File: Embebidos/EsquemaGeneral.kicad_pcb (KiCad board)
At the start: 2 copper layers, 100 x 99.9 mm, 79 parts, among them IC1 ESP32-WROVER-B__8MB_, J1 USB_A, J2 Conn_01x02, J3 RJ45, J4 RJ45, J5 Conn_02x06_Counter_Clockwise, J6 Conn_01x08, J7 Conn_01x04, Q1 BC847, Q2 BC847, Q3 BSS138, Q4 DMP3056LSDQ-13, Q5 BSS138, Q6 DMP3056LSDQ-13, SW1 SW_Reset, SW2 SW_Boot, U2 LM358, U3 SPX3819M5-L-3-3, U4 MIC29302WU, U5 MIC5219-3.3YM5

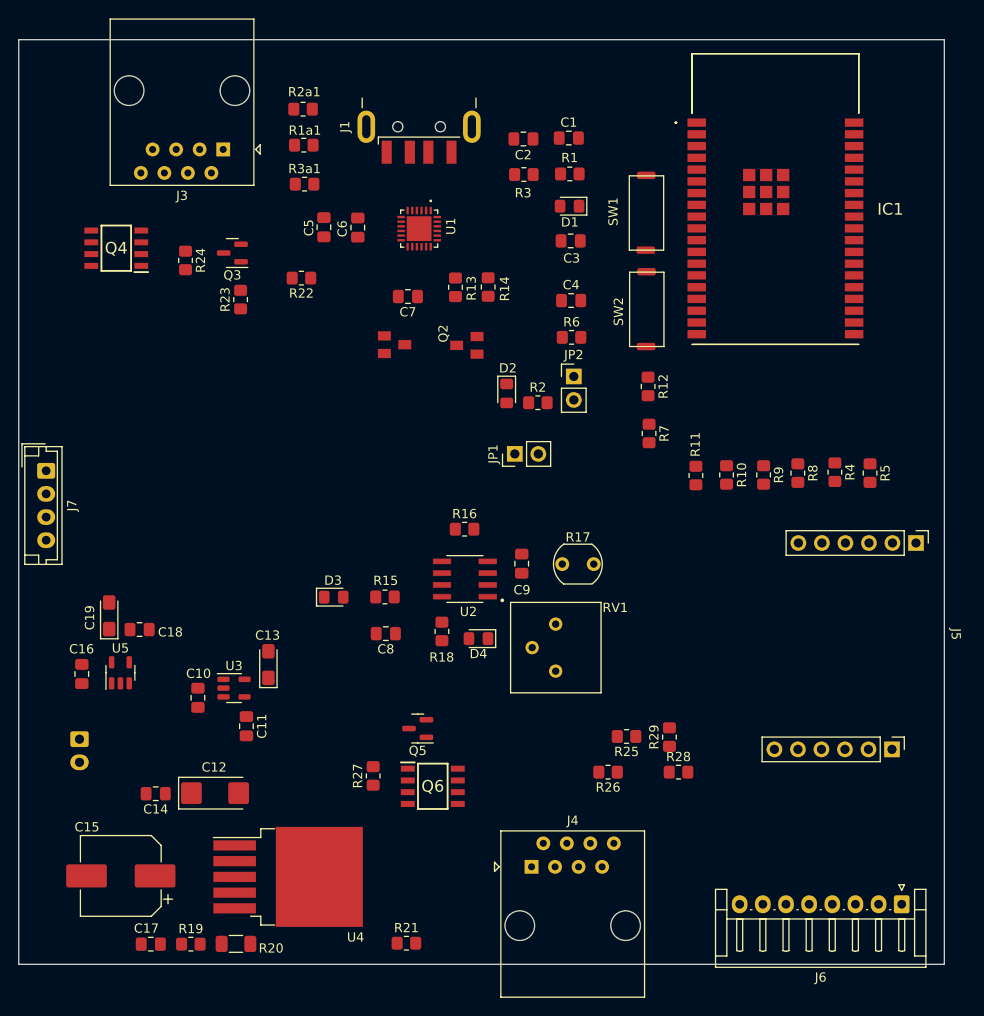
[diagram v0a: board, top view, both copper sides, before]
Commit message: pistas gordas :(
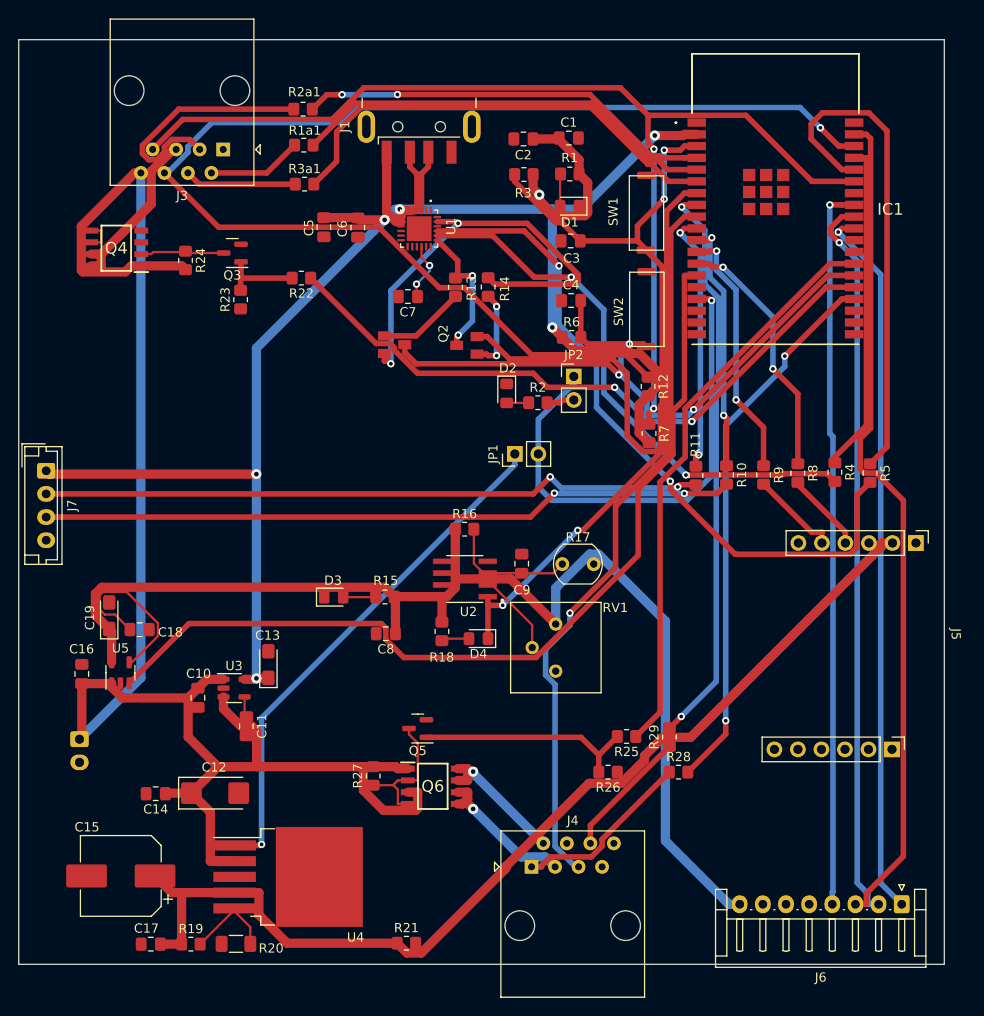
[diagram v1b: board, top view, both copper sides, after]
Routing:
- net +3.3V: track 0.00 -> 185.0 mm, vias 0 -> 7
- net +5V: track 0.00 -> 181.4 mm
- net /Acondicionamiento/SCL_PAN: track 0.00 -> 140.9 mm, vias 0 -> 1
- net 3.3Vop2: track 0.00 -> 129.0 mm
- net /Acondicionamiento/SDA_PAN: track 0.00 -> 116.6 mm, vias 0 -> 2
- net 4.1V: track 0.00 -> 111.3 mm
- net CtrlOnOff: track 0.00 -> 98.1 mm
- net /Acondicionamiento/MOSI_RFID: track 0.00 -> 90.7 mm
- net /Acondicionamiento/RESET: track 0.00 -> 83.9 mm, vias 0 -> 2
- net /Acondicionamiento/VO_Inf: track 0.00 -> 79.4 mm, vias 0 -> 1
- net /Acondicionamiento/SCK_RFID: track 0.00 -> 78.9 mm, vias 0 -> 1
- net /Acondicionamiento/MISO_RFID: track 0.00 -> 78.3 mm, vias 0 -> 1
- net /Acondicionamiento/CS_RFID: track 0.00 -> 77.3 mm, vias 0 -> 1
- net /Acondicionamiento/RXGPS: track 0.00 -> 75.0 mm, vias 0 -> 2
- net /Acondicionamiento/RXCP: track 0.00 -> 74.8 mm, vias 0 -> 2
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
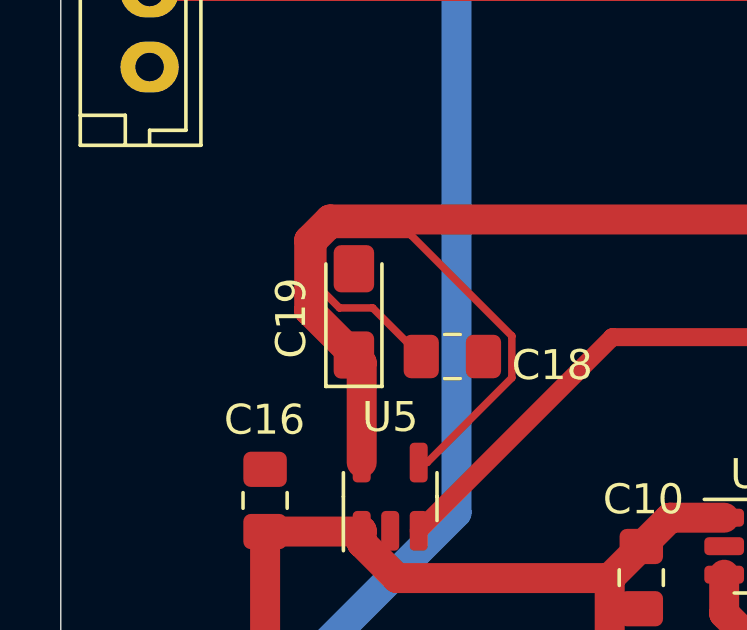
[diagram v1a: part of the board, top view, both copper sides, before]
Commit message: no se uwu
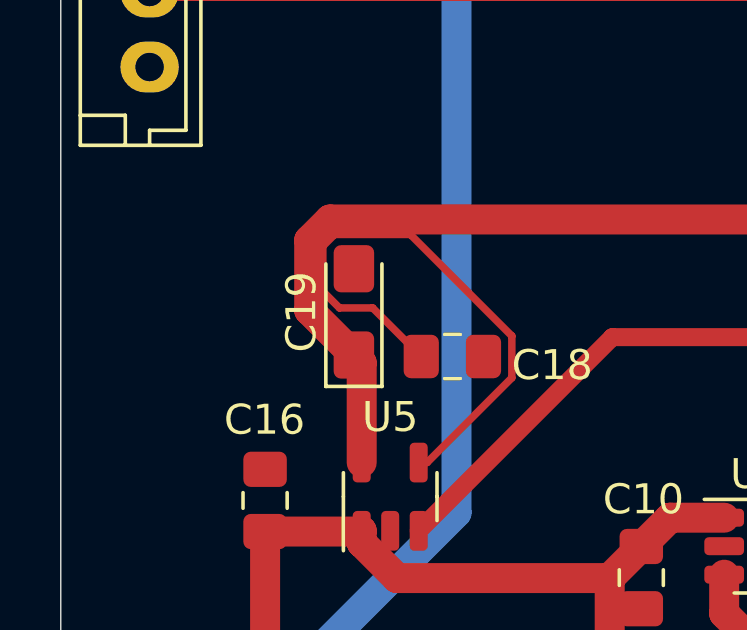
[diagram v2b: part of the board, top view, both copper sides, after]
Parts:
- C19: footprint Capacitor_Tantalum_SMD:CP_EIA-3216-12_Kemet-S_Pad1.58x1.35mm_HandSolder -> Capacitor_Tantalum_SMD:CP_EIA-3216-18_Kemet-A_Pad1.58x1.35mm_HandSolder
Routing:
- net +3.3V: track 185.0 -> 1457.2 mm, vias 7 -> 27
- net 4.1V: track 111.3 -> 322.6 mm, vias 0 -> 8
- net +5V: track 181.4 -> 0.00 mm
- net /Acondicionamiento/SCL_PAN: track 140.9 -> 0.00 mm, vias 1 -> 0
- net /Acondicionamiento/SDA_PAN: track 116.6 -> 0.00 mm, vias 2 -> 0
- net CtrlOnOff: track 98.1 -> 0.00 mm
- net Net-(IC1-Pad35): track 35.7 -> 126.3 mm
- net /Acondicionamiento/MOSI_RFID: track 90.7 -> 0.00 mm
- net /Acondicionamiento/RESET: track 83.9 -> 0.00 mm, vias 2 -> 0
- net /Acondicionamiento/VO_Inf: track 79.4 -> 0.00 mm, vias 1 -> 0
- net /Acondicionamiento/RXCP: track 74.8 -> 0.00 mm, vias 2 -> 0
- net /Acondicionamiento/GPIO0: track 74.3 -> 0.00 mm, vias 3 -> 0
- net /Acondicionamiento/Din_izq: track 61.9 -> 0.00 mm, vias 2 -> 0
- net /Acondicionamiento/LDR_IN: track 60.4 -> 0.00 mm, vias 2 -> 0
- net /Acondicionamiento/TXCP: track 59.3 -> 0.00 mm, vias 2 -> 0
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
